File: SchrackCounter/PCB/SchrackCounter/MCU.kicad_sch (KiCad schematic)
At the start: 3 parts, among them U7 ESP32-S3-WROOM-2

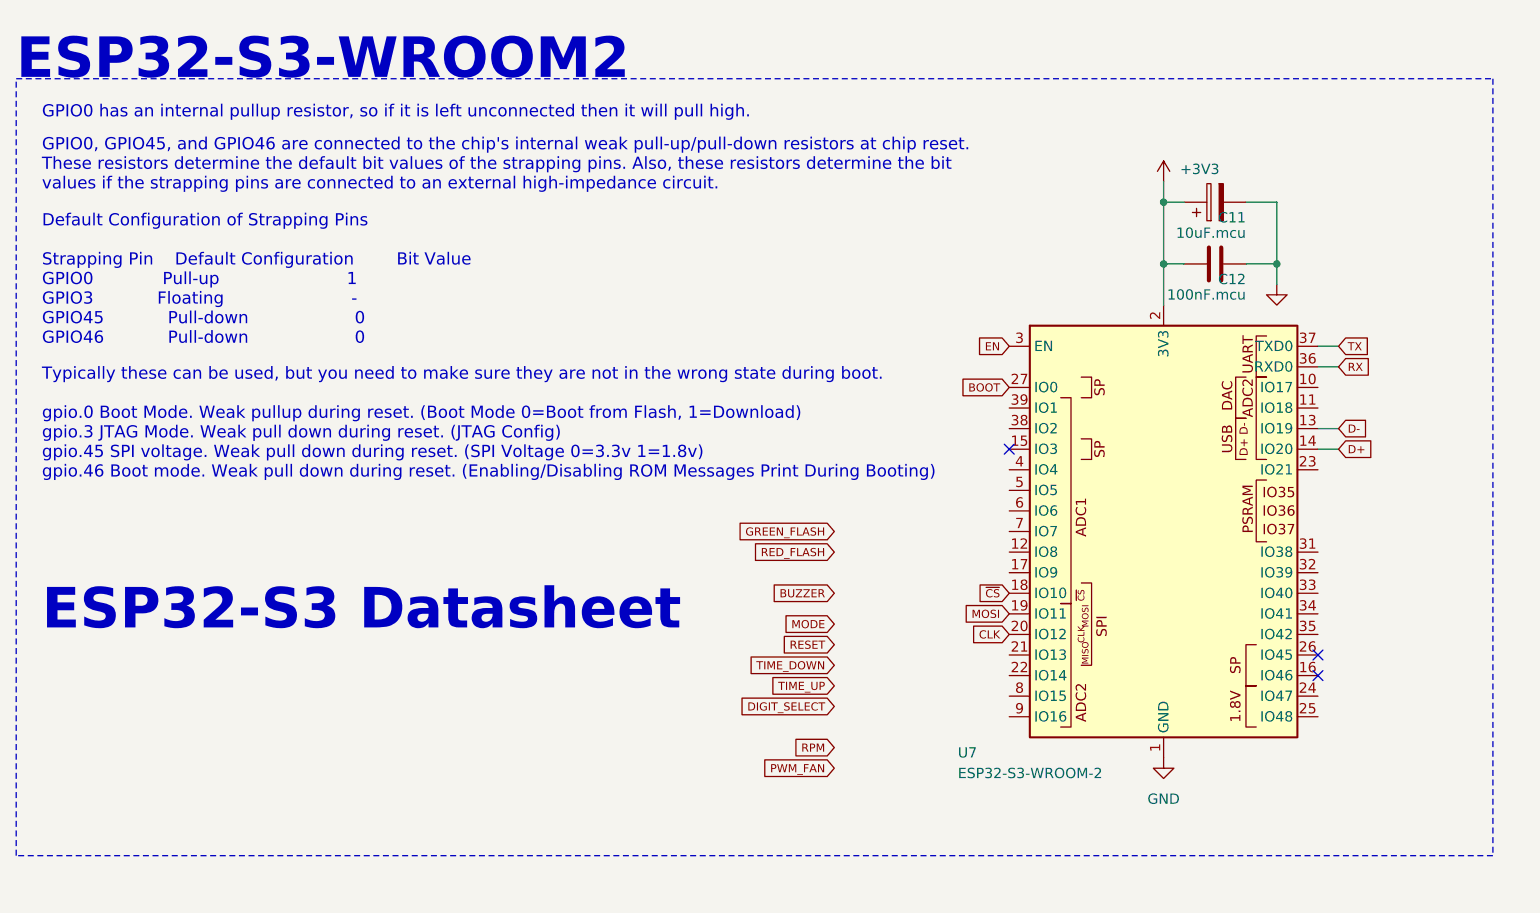
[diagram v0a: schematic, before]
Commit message: sleep, overated imo
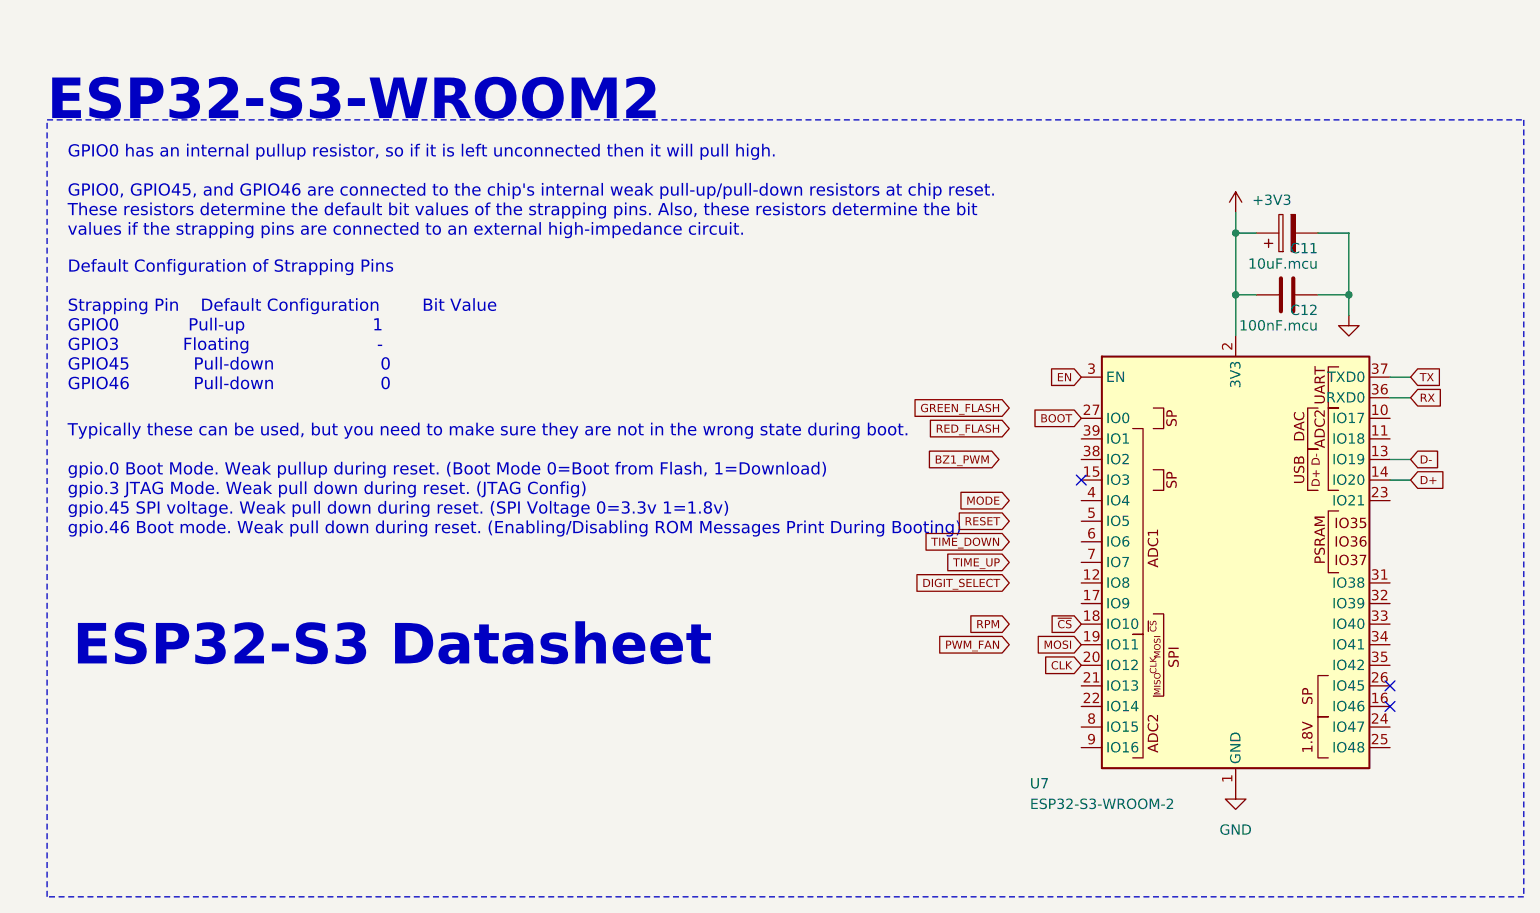
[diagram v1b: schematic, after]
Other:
- note added: "GPIO0 has an internal pullup resistor, so if it is left unconnected then it will pull high. GPIO0, GPIO45, and GPIO46 are connected to the chip's internal weak pull-up/pull-down resistors at chip reset. These resistors determine the default bit values of the strapping pins. Also, these resistors determine the bit values if the strapping pins are connected to an external high-impedance circuit."
- note removed: "GPIO0 has an internal pullup resistor, so if it is left unconnected then it will pull high."
- note removed: "GPIO0, GPIO45, and GPIO46 are connected to the chip's internal weak pull-up/pull-down resistors at chip reset. These resistors determine the default bit values of the strapping pins. Also, these resistors determine the bit values if the strapping pins are connected to an external high-impedance circuit."
- moved on the sheet: C11, C12, U7
